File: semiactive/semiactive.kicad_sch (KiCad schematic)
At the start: 1 part

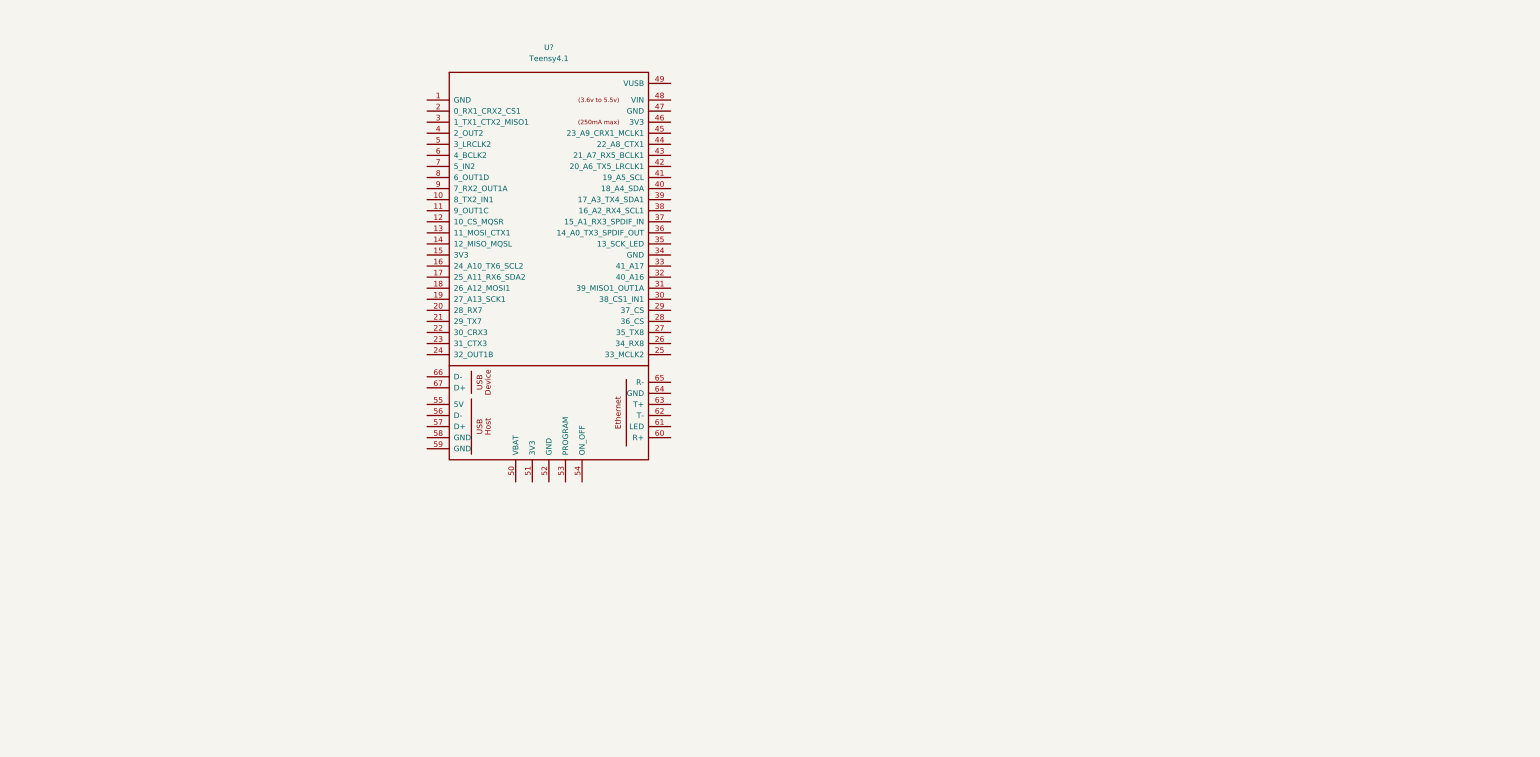
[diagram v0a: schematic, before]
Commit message: Setup libs, scripts
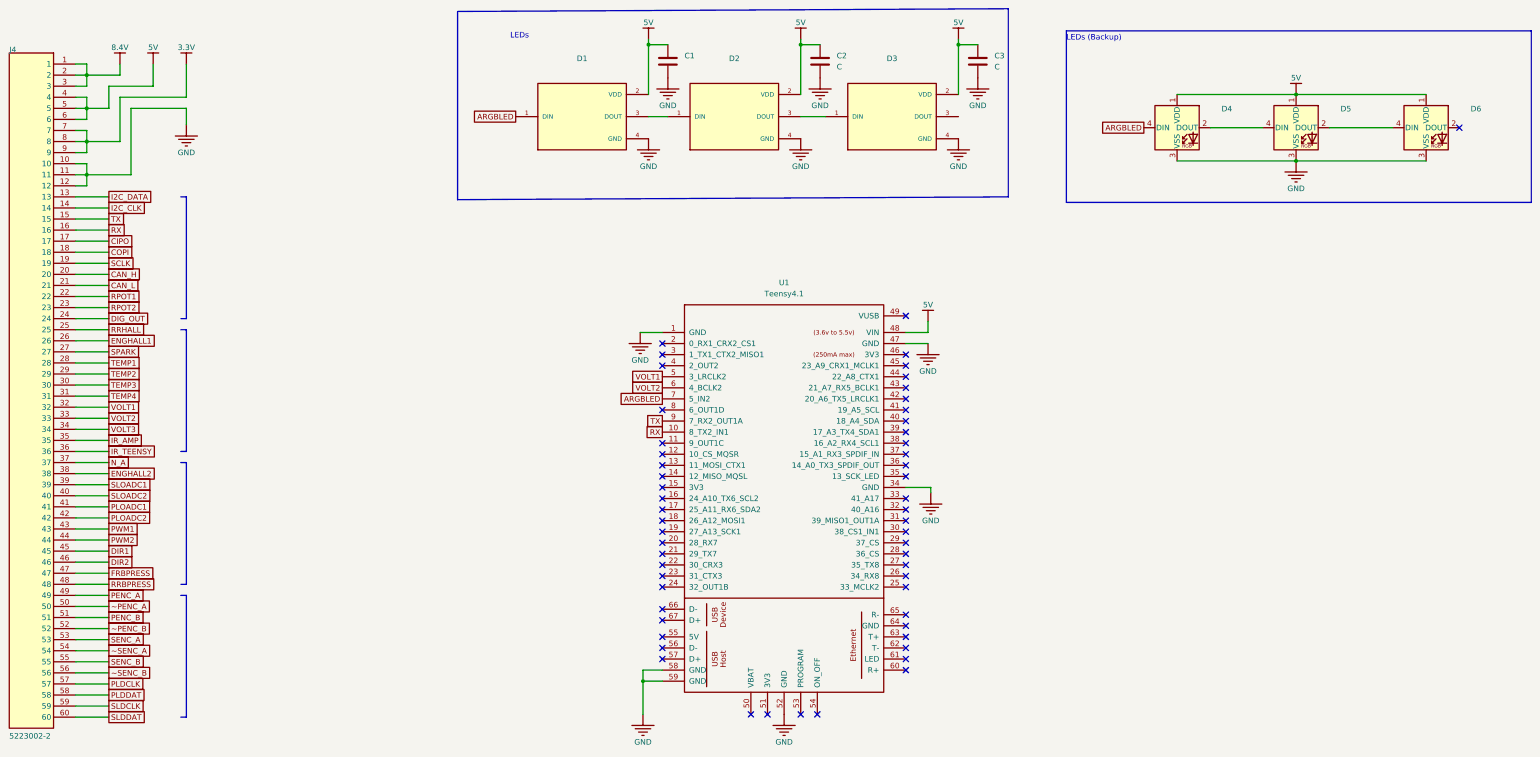
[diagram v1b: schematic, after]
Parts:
- removed U?: Teensy4.1, symbol teensy:Teensy4.1
- added C1: (no value), symbol Device:C
- added C2, C3: C, symbol Device:C
- added D1, D2, D3: (no value), symbol IN-PI42TASPRPGPB:IN-PI42TASPRPGPB
- added D4, D5, D6: (no value), symbol LED:WS2812B
- added J4: 5223002-2, symbol semiactive-altium-import:0_mirrored_5223002-2
- added U1: Teensy4.1, symbol teensy:Teensy4.1
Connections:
- new net: D2.3 (DOUT), D3.1 (DIN)
- new net: D4.2 (DOUT), D5.4 (DIN)
- new net: D1.3 (DOUT), D2.1 (DIN)
- new net: D5.2 (DOUT), D6.4 (DIN)
- new net 3.3V: J4.7, J4.8, J4.9
- new net 5V: C1.1, C2.1, C3.1, D1.2 (VDD), D2.2 (VDD), D3.2 (VDD), D4.1 (VDD), D5.1 (VDD), D6.1 (VDD), J4.4, J4.5, J4.6, U1.48 (VIN)
- new net 8.4V: J4.1, J4.2, J4.3
- new net ARGBLED: D1.1 (DIN), D4.4 (DIN), U1.7 (5_IN2)
- new net CAN_H: J4.20
- new net CAN_L: J4.21
- new net CIPO: J4.17
- new net COPI: J4.18
- new net DIG_OUT: J4.24
- new net DIR1: J4.45
- new net DIR2: J4.46
- new net ENGHALL1: J4.26
- new net ENGHALL2: J4.38
- new net FRBPRESS: J4.47
- new net GND: C1.2, C2.2, C3.2, D1.4 (GND), D2.4 (GND), D3.4 (GND), D4.3 (VSS), D5.3 (VSS), D6.3 (VSS), J4.10, J4.11, J4.12, U1.1 (GND), U1.34 (GND), U1.47 (GND), U1.52 (GND), U1.58 (GND), U1.59 (GND)
- new net I2C_CLK: J4.14
- new net I2C_DATA: J4.13
- new net IR_AMP: J4.35
- new net IR_TEENSY: J4.36
- new net N_A: J4.37
- new net PENC_A: J4.49
- new net PENC_B: J4.51
- new net PLDCLK: J4.57
- new net PLDDAT: J4.58
- new net PLOADC1: J4.41
- new net PLOADC2: J4.42
- new net PWM1: J4.43
- new net PWM2: J4.44
- new net RPOT1: J4.22
- new net RPOT2: J4.23
- new net RRBPRESS: J4.48
- new net RRHALL: J4.25
- new net RX: J4.16, U1.10 (8_TX2_IN1)
- new net SCLK: J4.19
- new net SENC_A: J4.53
- new net SENC_B: J4.55
- new net SLDCLK: J4.59
- new net SLDDAT: J4.60
- new net SLOADC1: J4.39
- new net SLOADC2: J4.40
- new net SPARK: J4.27
- new net TEMP1: J4.28
- new net TEMP2: J4.29
- new net TEMP3: J4.30
- new net TEMP4: J4.31
- new net TX: J4.15, U1.9 (7_RX2_OUT1A)
- new net VOLT1: J4.32, U1.5 (3_LRCLK2)
- new net VOLT2: J4.33, U1.6 (4_BCLK2)
- new net VOLT3: J4.34
- new net ~PENC_A: J4.50
- new net ~PENC_B: J4.52
- new net ~SENC_A: J4.54
- new net ~SENC_B: J4.56
- no-connect marks 0 -> 56
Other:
- note added: "LEDs"
- note added: "LEDs (Backup)"

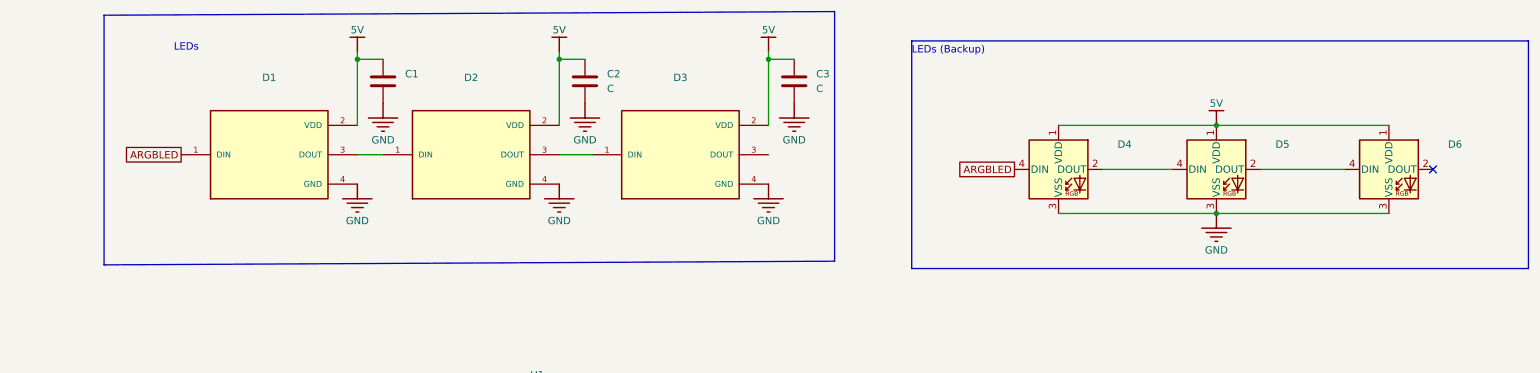
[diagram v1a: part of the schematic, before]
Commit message: Create a few projects
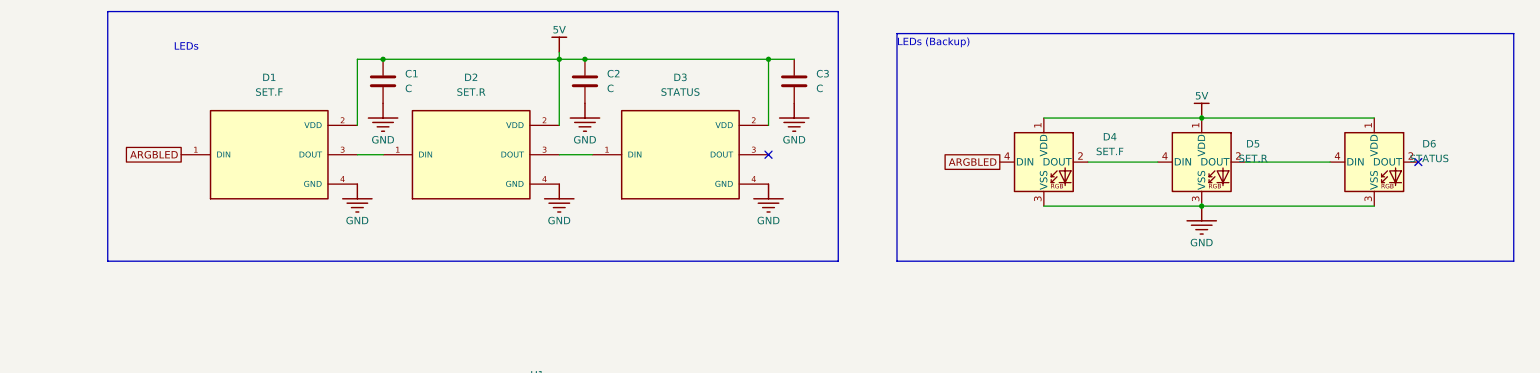
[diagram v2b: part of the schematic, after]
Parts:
- C1: value (none) -> C; footprint (none) -> Capacitor_SMD:C_0603_1608Metric
- C2, C3: footprint (none) -> Capacitor_SMD:C_0603_1608Metric
- D1: value (none) -> SET.F; footprint (none) -> !footprints:LED_IN-PI42TASPRPGPB
- D2: value (none) -> SET.R; footprint (none) -> !footprints:LED_IN-PI42TASPRPGPB
- D3: value (none) -> STATUS; footprint (none) -> !footprints:LED_IN-PI42TASPRPGPB
- D4: value (none) -> SET.F; footprint (none) -> !footprints:LED_WS2812B_PLCC4_5.0x5.0mm_P3.2mm
- D5: value (none) -> SET.R; footprint (none) -> !footprints:LED_WS2812B_PLCC4_5.0x5.0mm_P3.2mm
- D6: value (none) -> STATUS; footprint (none) -> !footprints:LED_WS2812B_PLCC4_5.0x5.0mm_P3.2mm
- J4: footprint (none) -> !footprints:52230042
- U1: footprint (none) -> !footprints:Teensy41
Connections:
- no-connect marks 56 -> 57
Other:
- moved on the sheet: D4, D5, D6
